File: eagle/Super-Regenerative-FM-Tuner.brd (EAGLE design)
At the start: 45.7 x 20.3 mm, 14 parts, among them T1 BF245BTO92

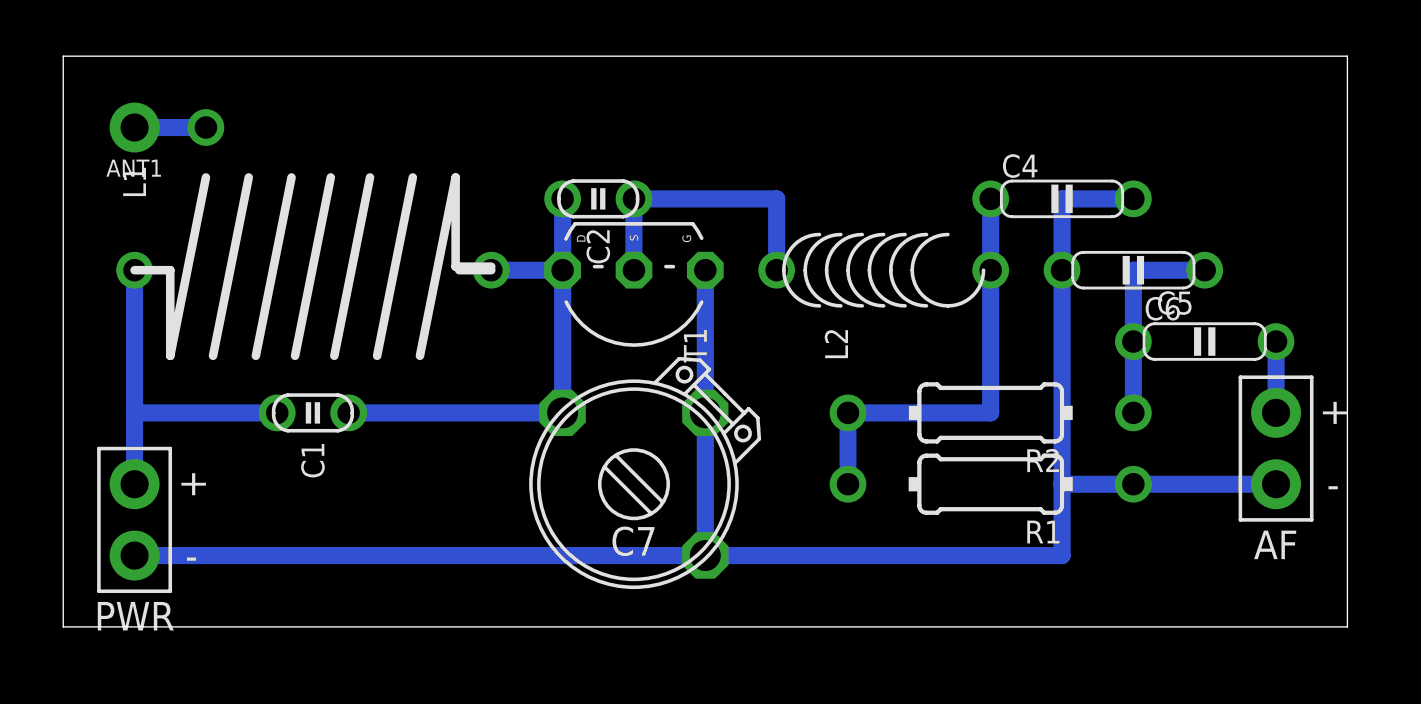
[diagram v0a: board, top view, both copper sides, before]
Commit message: ...
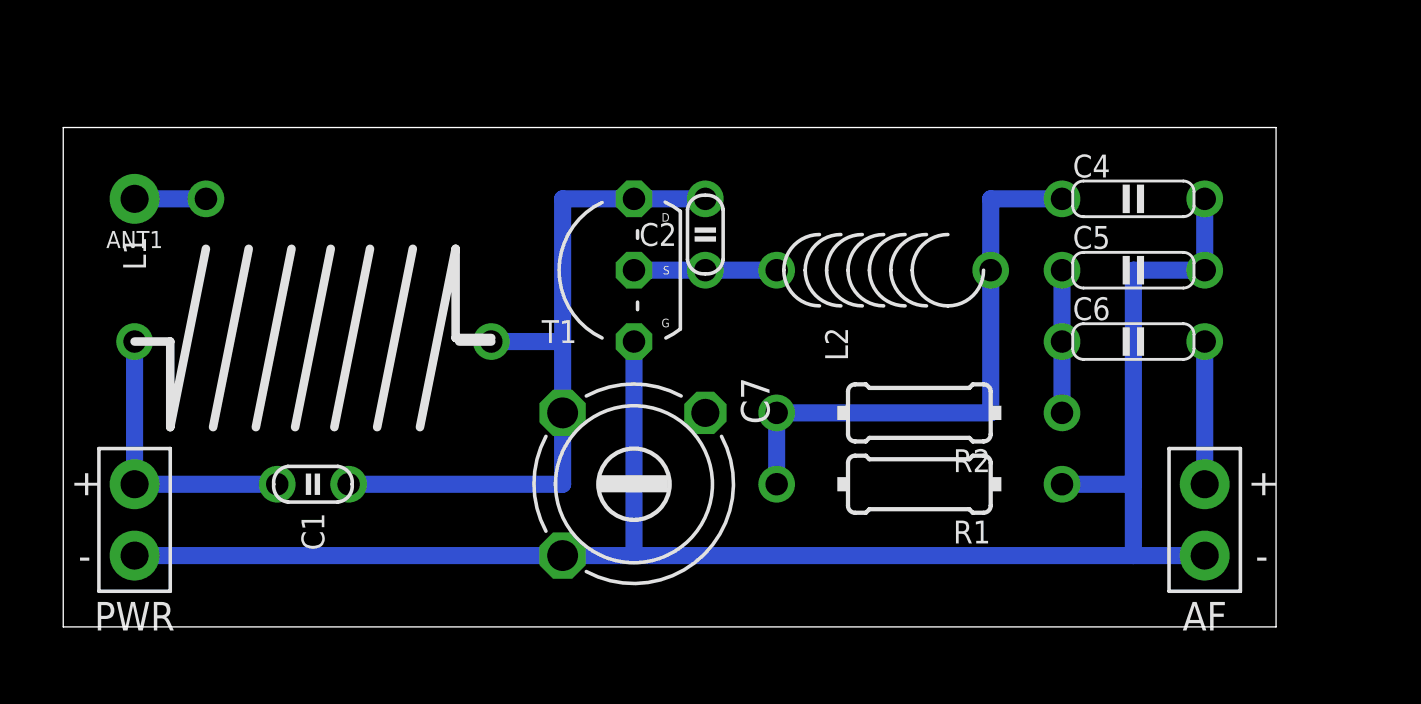
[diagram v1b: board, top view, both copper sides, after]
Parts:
- AF: value SPAD+- -> SPAD+-+-
- C7: device cap-trim:TRIM-2222-808 -> cap-trim:TRIM808-45
- PWR: device pad:SPAD+- -> pad:SPAD-+
- T1: value BF245BTO92 -> BF245A
- moved C2 4.02 mm to (22.9, 14.0), turned to 0 degrees
- moved AF 3.59 mm to (40.6, 3.81)
- moved R1 2.54 mm to (30.5, 5.08)
- moved R2 2.54 mm to (30.5, 7.62)
- moved ANT1 2.54 mm to (2.54, 15.2)
- moved C1 2.54 mm to (8.89, 5.08)
- moved C4 2.54 mm to (38.1, 15.2)
- moved C6 2.54 mm to (38.1, 10.2)
- moved L1 2.54 mm to (8.89, 10.2)
- turned C5 to 0 degrees
- turned C7 to 270 degrees
- turned T1 to 180 degrees
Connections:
- net GND: now also C7.1; no longer C7.2
- net N$1: now also C7.2; no longer C7.3
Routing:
- net N$1: track 17.8 -> 25.4 mm
- net N$5: track 10.2 -> 5.08 mm
- net N$2: track 15.2 -> 20.3 mm
- net N$8: track 2.54 -> 5.08 mm
- net VCC: track 12.7 -> 10.2 mm
- net N$6: track 7.62 -> 5.08 mm
- net GND: track 66.0 -> 63.5 mm
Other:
- board size 45.7 x 20.3 mm -> 43.2 x 17.8 mm
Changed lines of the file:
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@@
 <board>
 <plain>
-<wire x1="45.72" y1="0" x2="45.72" y2="20.32" width="0" layer="20"/>
-<wire x1="45.72" y1="20.32" x2="0" y2="20.32" width="0" layer="20"/>
-<wire x1="0" y1="20.32" x2="0" y2="0" width="0" layer="20"/>
-<wire x1="0" y1="0" x2="45.72" y2="0" width="0" layer="20"/>
+<wire x1="43.18" y1="0" x2="43.18" y2="17.78" width="0" layer="20"/>
+<wire x1="43.18" y1="17.78" x2="0" y2="17.78" width="0" layer="20"/>
+<wire x1="0" y1="17.78" x2="0" y2="0" width="0" layer="20"/>
+<wire x1="0" y1="0" x2="43.18" y2="0" width="0" layer="20"/>
 </plain>
 <attributes>
@@
 </autorouter>
 <elements>
-<element name="AF" library="pad" package="SPAD+-" value="SPAD+-" x="43.18" y="6.35"/>
-<element name="ANT1" library="pad" package="SPAD" value="ANT" x="2.54" y="17.78" rot="R90"/>
-<element name="C1" library="c" package="C025-015X024" value="20pF" x="8.89" y="7.62" rot="R90"/>
-<element name="C2" library="c" package="C025-015X024" value="10pF" x="19.05" y="15.24" rot="R90"/>
-<element name="C4" library="c" package="C050-020X044" value="2.7nF" x="35.56" y="15.24"/>
-<element name="C5" library="c" package="C050-020X044" value="10nF" x="38.1" y="12.7" rot="R180"/>
-<element name="C6" library="c" package="C050-020X044" value="100nF" x="40.64" y="10.16"/>
-<element name="C7" library="cap-trim" package="TRIM-2222-808" value="0.04 - 6pF" x="20.32" y="5.08" rot="R180"/>
-<element name="PWR" library="pad" package="SPAD+-" value="" x="2.54" y="3.81"/>
-<element name="L1" library="l" package="L-08/10V-TAP1" value="*" x="8.89" y="12.7" rot="R90"/>
+<element name="AF" library="pad" package="SPAD+-" value="SPAD+-+-" x="40.64" y="3.81"/>
+<element name="ANT1" library="pad" package="SPAD" value="ANT" x="2.54" y="15.24" rot="R90"/>
+<element name="C1" library="c" package="C025-015X024" value="20pF" x="8.89" y="5.08" rot="R90"/>
+<element name="C2" library="c" package="C025-015X024" value="10pF" x="22.86" y="13.97"/>
+<element name="C4" library="c" package="C050-020X044" value="2.7nF" x="38.1" y="15.24"/>
+<element name="C5" library="c" package="C050-020X044" value="10nF" x="38.1" y="12.7"/>
+<element name="C6" library="c" package="C050-020X044" value="100nF" x="38.1" y="10.16"/>
+<element name="C7" library="cap-trim" package="TRIM808-45" value="0.04 - 6pF" x="20.32" y="5.08" rot="R270"/>
+<element name="L1" library="l" package="L-08/10V-TAP1" value="*" x="8.89" y="10.16" rot="R90"/>
 <element name="L2" library="l" package="L-04/7-V" value="8.2uH" x="29.21" y="12.7" rot="R90"/>
-<element name="R1" library="r" package="0204/10-V" value="10k" x="33.02" y="5.08" rot="R90"/>
-<element name="R2" library="r" package="0204/10-V" value="12k" x="33.02" y="7.62" rot="R90"/>
-<element name="T1" library="t" package="TO92-GSD" value="BF245BTO92" x="20.32" y="12.7" rot="R270"/>
+<element name="R1" library="r" package="0204/10-V" value="10k" x="30.48" y="5.08" rot="R90"/>
+<element name="R2" library="r" package="0204/10-V" value="12k" x="30.48" y="7.62" rot="R90"/>
+<element name="T1" library="t" package="TO92-GSD" value="BF245A" x="20.32" y="12.7" rot="R180"/>
+<element name="PWR" library="pad" package="SPAD-+" value="" x="2.54" y="3.81"/>
 </elements>
 <signals>
@@
 <contactref element="L1" pad="2"/>
 <contactref element="C1" pad="2"/>
-<contactref element="C7" pad="3"/>
-<wire x1="17.78" y1="12.7" x2="17.78" y2="7.62" width="0.6096" layer="16"/>
-<wire x1="15.24" y1="12.7" x2="17.78" y2="12.7" width="0.6096" layer="16"/>
-<wire x1="17.78" y1="15.24" x2="17.78" y2="12.7" width="0.6096" layer="16"/>
-<wire x1="10.16" y1="7.62" x2="17.78" y2="7.62" width="0.6096" layer="16"/>
+<contactref element="C7" pad="2"/>
+<wire x1="17.78" y1="10.16" x2="17.78" y2="7.62" width="0.6096" layer="16"/>
+<wire x1="15.24" y1="10.16" x2="17.78" y2="10.16" width="0.6096" layer="16"/>
+<wire x1="17.78" y1="10.16" x2="17.78" y2="15.24" width="0.6096" layer="16"/>
+<wire x1="17.78" y1="15.24" x2="20.32" y2="15.24" width="0.6096" layer="16"/>
+<wire x1="22.86" y1="15.24" x2="20.32" y2="15.24" width="0.6096" layer="16"/>
+<wire x1="10.16" y1="5.08" x2="17.78" y2="5.08" width="0.6096" layer="16"/>
+<wire x1="17.78" y1="5.08" x2="17.78" y2="7.62" width="0.6096" layer="16"/>
 </signal>
 <signal name="N$4">
 <contactref element="L1" pad="3"/>
 <contactref element="ANT1" pad="1"/>
-<wire x1="2.54" y1="17.78" x2="5.08" y2="17.78" width="0.6096" layer="16"/>
+<wire x1="2.54" y1="15.24" x2="5.08" y2="15.24" width="0.6096" layer="16"/>
 </signal>
 <signal name="N$5">
@@
 <contactref element="C2" pad="2"/>
 <contactref element="L2" pad="1"/>
-<wire x1="20.32" y1="15.24" x2="25.4" y2="15.24" width="0.6096" layer="16"/>
-<wire x1="25.4" y1="15.24" x2="25.4" y2="12.7" width="0.6096" layer="16"/>
-<wire x1="20.32" y1="12.7" x2="20.32" y2="15.24" width="0.6096" layer="16"/>
+<wire x1="22.86" y1="12.7" x2="25.4" y2="12.7" width="0.6096" layer="16"/>
+<wire x1="20.32" y1="12.7" x2="22.86" y2="12.7" width="0.6096" layer="16"/>
 </signal>
 <signal name="GND">
 <contactref element="T1" pad="1"/>
-<contactref element="C7" pad="2"/>
+<contactref element="C7" pad="1"/>
 <contactref element="AF" pad="1"/>
+<wire x1="20.32" y1="2.54" x2="38.1" y2="2.54" width="0.6096" layer="16"/>
 <contactref element="C4" pad="2"/>
 <contactref element="R1" pad="2"/>
 <contactref element="C5" pad="2"/>
 <contactref element="PWR" pad="1"/>
-<wire x1="22.86" y1="2.54" x2="35.56" y2="2.54" width="0.6096" layer="16"/>
-<wire x1="35.56" y1="2.54" x2="35.56" y2="5.08" width="0.6096" layer="16"/>
-<wire x1="2.54" y1="2.54" x2="22.86" y2="2.54" width="0.6096" layer="16"/>
-<wire x1="22.86" y1="12.7" x2="22.86" y2="7.62" width="0.6096" layer="16"/>
-<wire x1="22.86" y1="7.62" x2="22.86" y2="2.54" width="0.6096" layer="16"/>
-<wire x1="35.56" y1="12.7" x2="35.56" y2="5.08" width="0.6096" layer="16"/>
-<wire x1="35.56" y1="5.08" x2="38.1" y2="5.08" width="0.6096" layer="16"/>
-<wire x1="38.1" y1="15.24" x2="35.56" y2="15.24" width="0.6096" layer="16"/>
-<wire x1="35.56" y1="15.24" x2="35.56" y2="12.7" width="0.6096" layer="16"/>
-<wire x1="38.1" y1="5.08" x2="43.18" y2="5.08" width="0.6096" layer="16"/>
+<wire x1="40.64" y1="15.24" x2="40.64" y2="12.7" width="0.6096" layer="16"/>
+<wire x1="17.78" y1="2.54" x2="2.54" y2="2.54" width="0.6096" layer="16"/>
+<wire x1="40.64" y1="2.54" x2="38.1" y2="2.54" width="0.6096" layer="16"/>
+<wire x1="38.1" y1="2.54" x2="38.1" y2="5.08" width="0.6096" layer="16"/>
+<wire x1="40.64" y1="12.7" x2="38.1" y2="12.7" width="0.6096" layer="16"/>
+<wire x1="38.1" y1="12.7" x2="38.1" y2="5.08" width="0.6096" layer="16"/>
+<wire x1="38.1" y1="5.08" x2="35.56" y2="5.08" width="0.6096" layer="16"/>
+<wire x1="20.32" y1="10.16" x2="20.32" y2="2.54" width="0.6096" layer="16"/>
+<wire x1="20.32" y1="2.54" x2="17.78" y2="2.54" width="0.6096" layer="16"/>
 </signal>
 <signal name="N$2">
@@
 <contactref element="L2" pad="2"/>
 <contactref element="R1" pad="1"/>
-<wire x1="33.02" y1="7.62" x2="27.94" y2="7.62" width="0.6096" layer="16"/>
-<wire x1="27.94" y1="7.62" x2="27.94" y2="5.08" width="0.6096" layer="16"/>
+<wire x1="33.02" y1="7.62" x2="25.4" y2="7.62" width="0.6096" layer="16"/>
+<wire x1="25.4" y1="7.62" x2="25.4" y2="5.08" width="0.6096" layer="16"/>
+<wire x1="35.56" y1="15.24" x2="33.02" y2="15.24" width="0.6096" layer="16"/>
 <wire x1="33.02" y1="15.24" x2="33.02" y2="12.7" width="0.6096" layer="16"/>
 <wire x1="33.02" y1="7.62" x2="33.02" y2="12.7" width="0.6096" layer="16"/>
@@
 <contactref element="C5" pad="1"/>
 <contactref element="C6" pad="1"/>
-<wire x1="38.1" y1="7.62" x2="38.1" y2="10.16" width="0.6096" layer="16"/>
-<wire x1="40.64" y1="12.7" x2="38.1" y2="12.7" width="0.6096" layer="16"/>
-<wire x1="38.1" y1="12.7" x2="38.1" y2="10.16" width="0.6096" layer="16"/>
+<wire x1="35.56" y1="7.62" x2="35.56" y2="10.16" width="0.6096" layer="16"/>
+<wire x1="35.56" y1="12.7" x2="35.56" y2="10.16" width="0.6096" layer="16"/>
 </signal>
 <signal name="N$8">
 <contactref element="C6" pad="2"/>
 <contactref element="AF" pad="2"/>
-<wire x1="43.18" y1="7.62" x2="43.18" y2="10.16" width="0.6096" layer="16"/>
+<wire x1="40.64" y1="5.08" x2="40.64" y2="10.16" width="0.6096" layer="16"/>
 </signal>
 <signal name="VCC">
@@
 <contactref element="L1" pad="1"/>
 <contactref element="PWR" pad="2"/>
-<wire x1="2.54" y1="5.08" x2="2.54" y2="7.62" width="0.6096" layer="16"/>
-<wire x1="2.54" y1="7.62" x2="7.62" y2="7.62" width="0.6096" layer="16"/>
-<wire x1="2.54" y1="12.7" x2="2.54" y2="7.62" width="0.6096" layer="16"/>
+<wire x1="2.54" y1="5.08" x2="7.62" y2="5.08" width="0.6096" layer="16"/>
+<wire x1="2.54" y1="10.16" x2="2.54" y2="5.08" width="0.6096" layer="16"/>
 </signal>
 </signals>
